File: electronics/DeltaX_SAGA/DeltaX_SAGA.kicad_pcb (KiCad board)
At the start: 4 copper layers, 76 parts, among them J1 USB_B_Micro, J10 Motor3_Encoder, J11 M12, J12 M21, J13 M22, J14 M31, J15 M33, J16 Thrower+, J17 Thrower-, J2 Programmer, J3 SERVO, J4 M11, J5 Battery+, J6 Thrower Signal, J7 Battery-, J8 Motor1_Encoder, J9 Motor2_Encoder, Q1 BUK6Y10, U1 CM1223, U10 DRV8243, U11 DRV8243, U2 NCP164C, U3 STM32G441KB, U4 NCV8730, U5 TPS62933, U6 MAX14930, U7 MAX14930, U8 MAX12930, U9 DRV8243

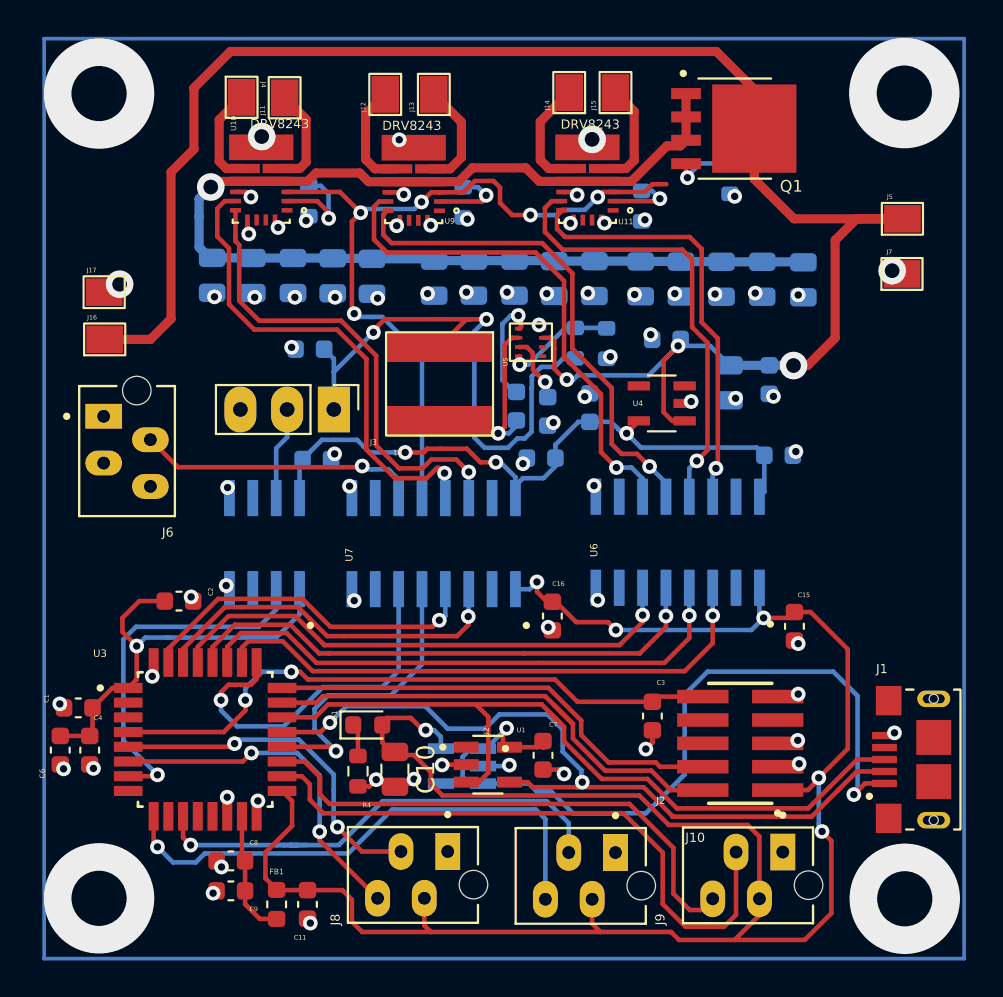
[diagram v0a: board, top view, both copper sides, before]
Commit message: complete PCB updated
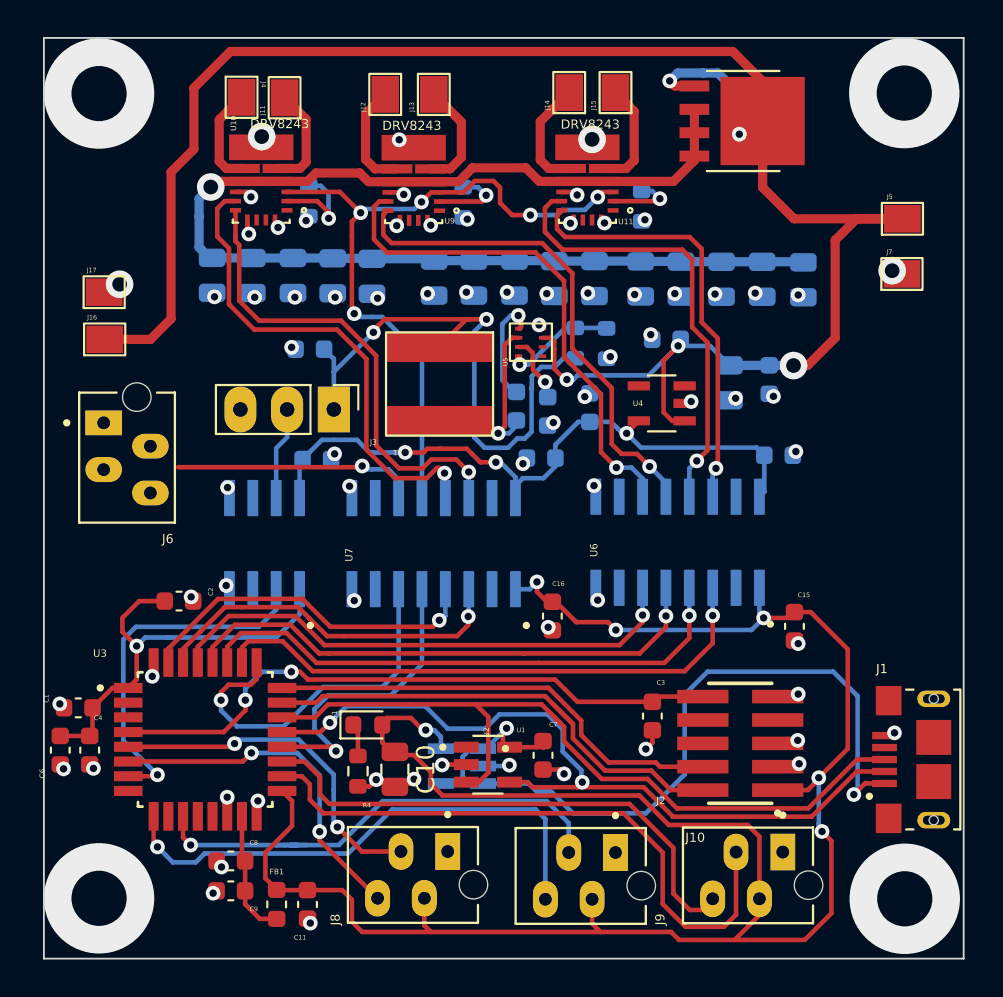
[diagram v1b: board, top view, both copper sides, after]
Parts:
- Q1: moved to F.Cu
- moved R3 3.39 mm to (163.5, 87.0)
- moved Q1 1.50 mm to (164.0, 86.7), turned to -90 degrees
- moved J6 0.36 mm to (129.2, 103.6)
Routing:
- net /nSLEEP_Isolated: track 41.8 -> 38.8 mm
- net Net-(Q1-Pad4): track 3.47 -> 6.17 mm
- net /Thrower_PWM_Isolated: track 15.4 -> 13.3 mm
- net /V+: track 97.7 -> 98.3 mm
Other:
- board outline added: 50 x 50 mm
